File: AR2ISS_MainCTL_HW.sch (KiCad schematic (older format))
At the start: 3 parts

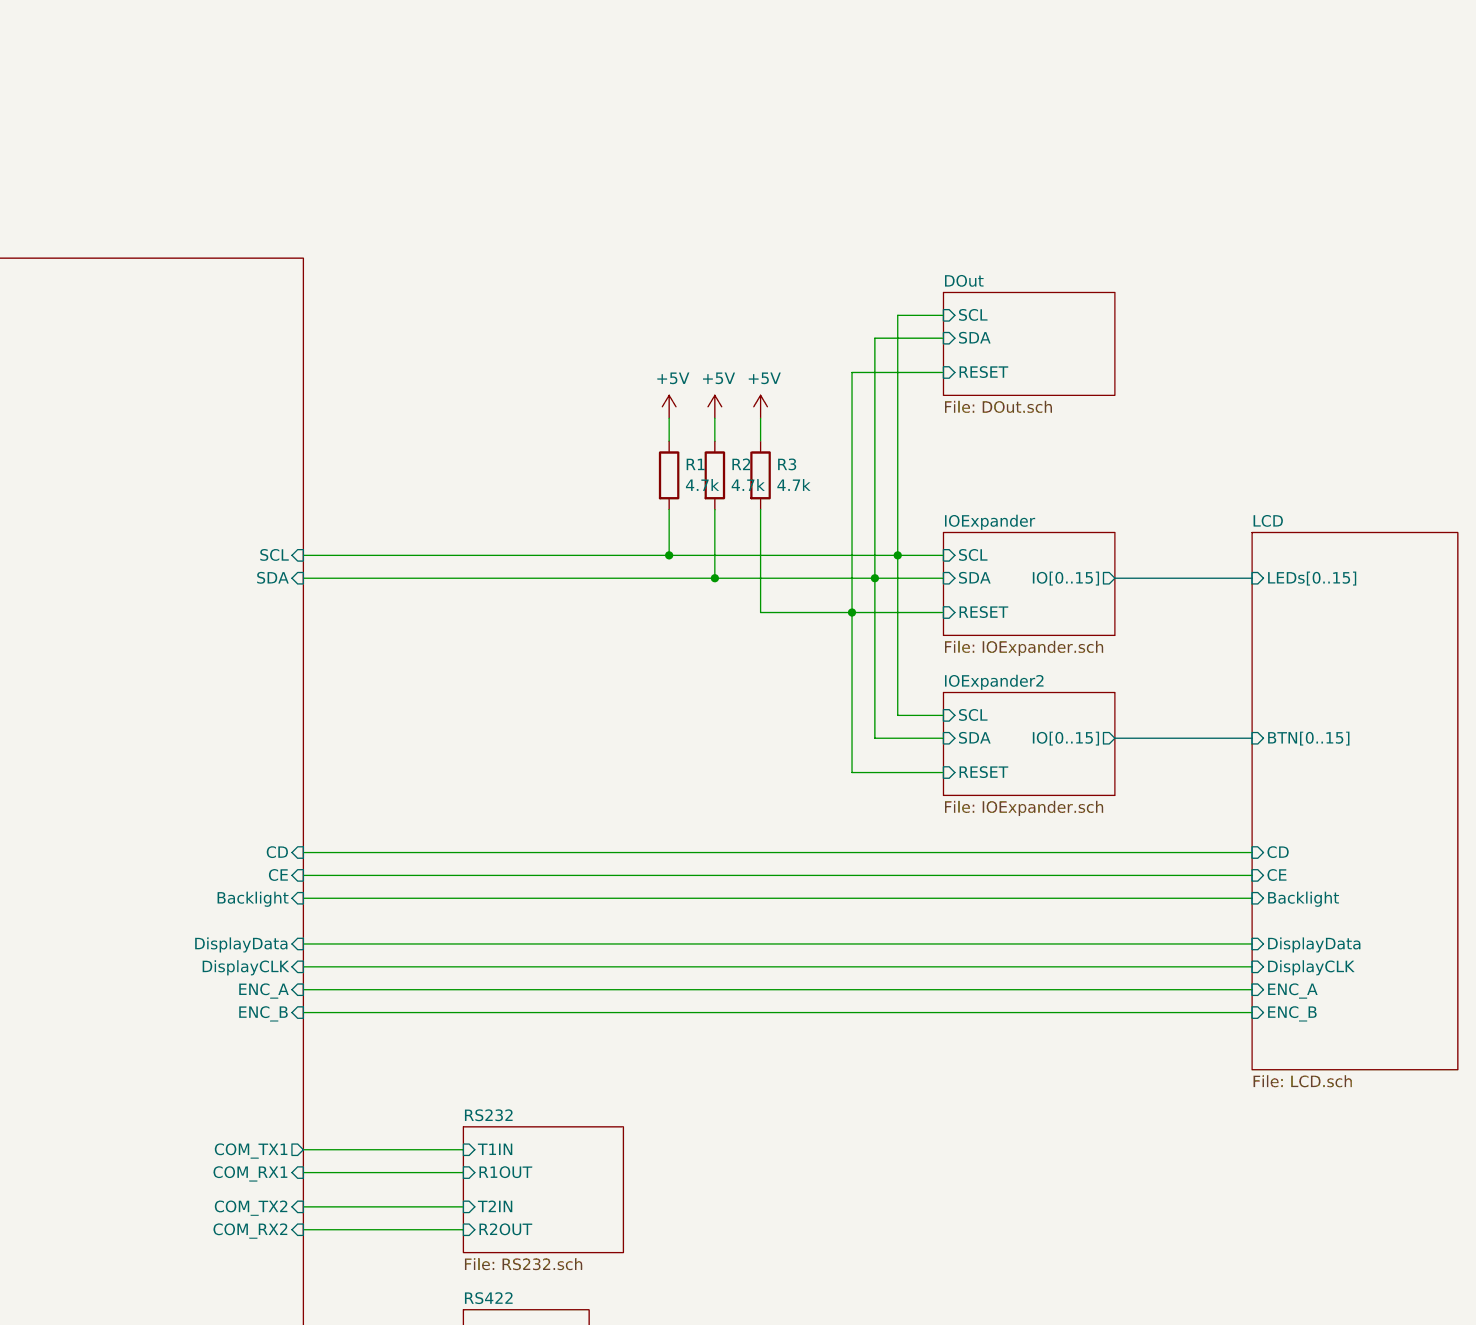
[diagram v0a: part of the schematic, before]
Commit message: placement, routing
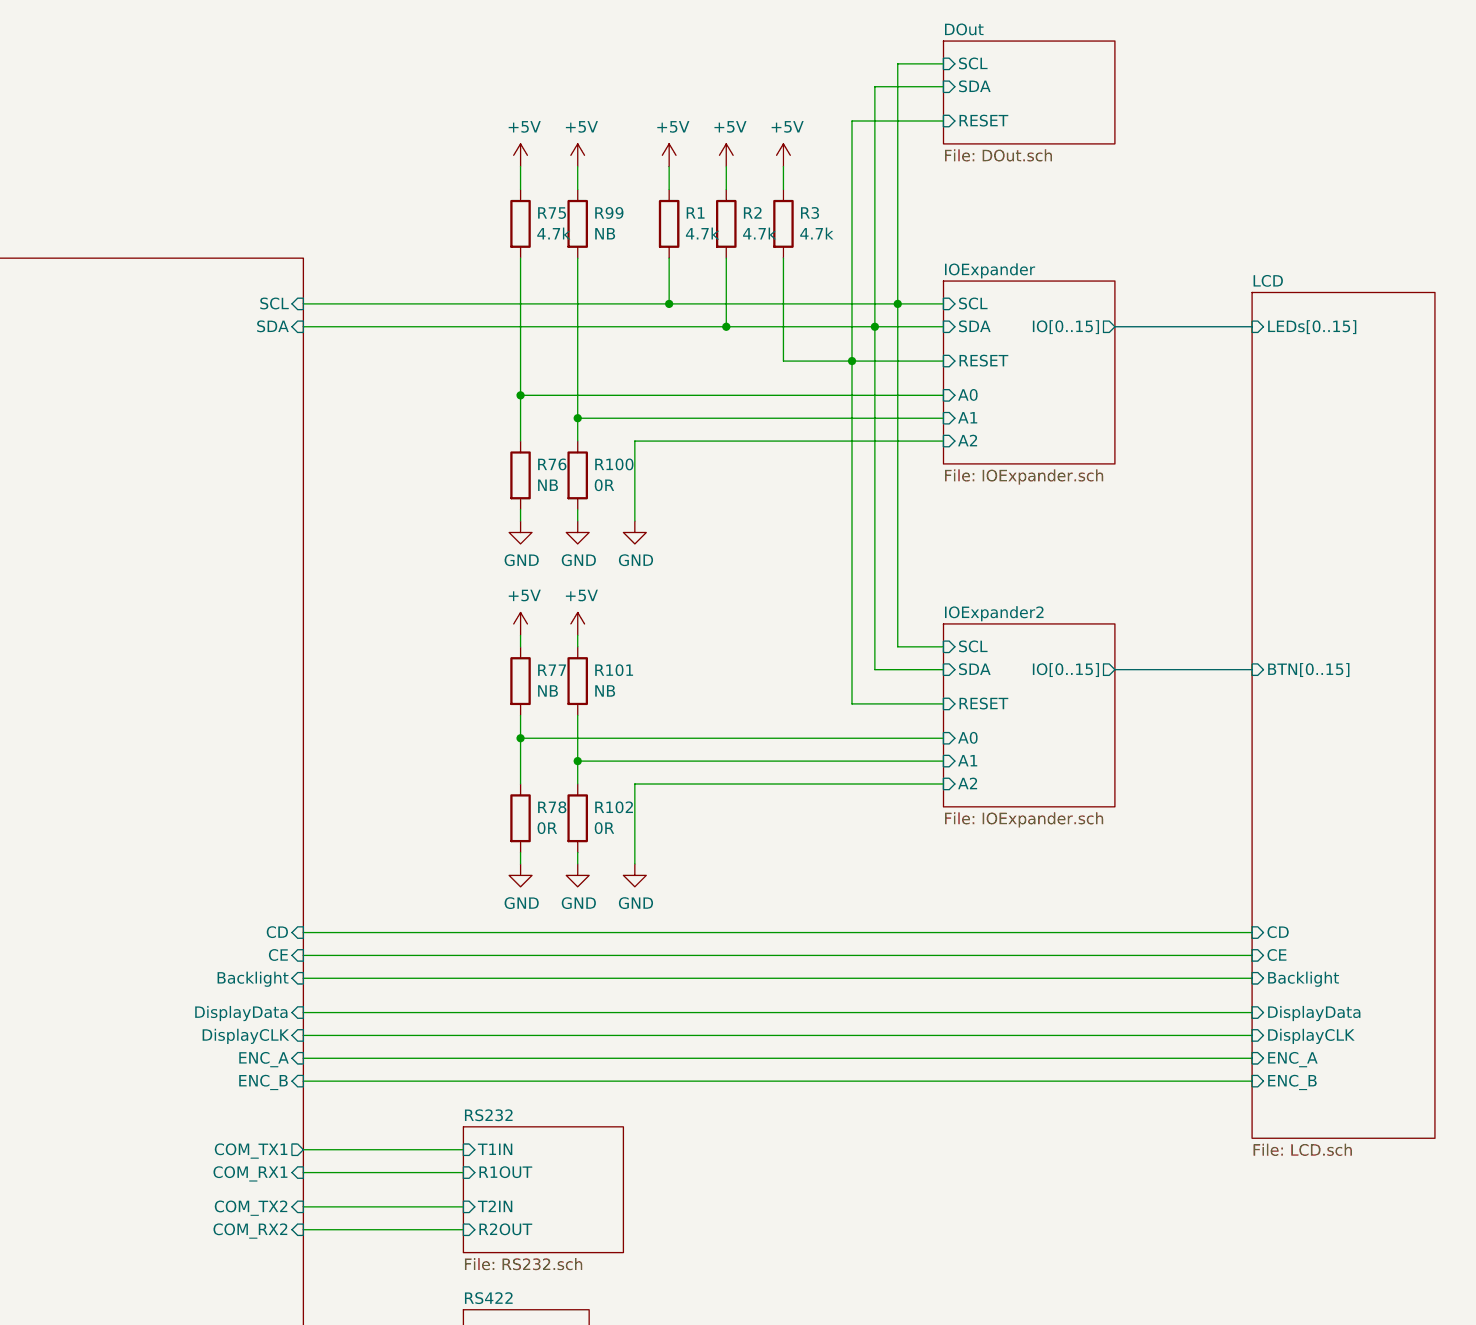
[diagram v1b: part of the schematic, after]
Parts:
- added R100, R102, R78: 0R, Resistor_SMD:R_0603_1608Metric, symbol AR2ISS:R
- added R101, R76, R77, R99: NB, Resistor_SMD:R_0603_1608Metric, symbol AR2ISS:R
- added R75: 4.7k, Resistor_SMD:R_0603_1608Metric, symbol AR2ISS:R
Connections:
- net +5V: now also R101.1, R75.1, R77.1, R99.1
- new net GND: R100.2, R102.2, R76.2, R78.2
- new net IOExpander/A0: R75.2, R76.1
- new net IOExpander/A1: R100.1, R99.2
- new net IOExpander2/A0: R77.2, R78.1
- new net IOExpander2/A1: R101.2, R102.1
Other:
- moved on the sheet: R1, R2, R3
